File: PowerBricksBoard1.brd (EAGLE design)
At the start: 75.6 x 50.8 mm, 16 parts

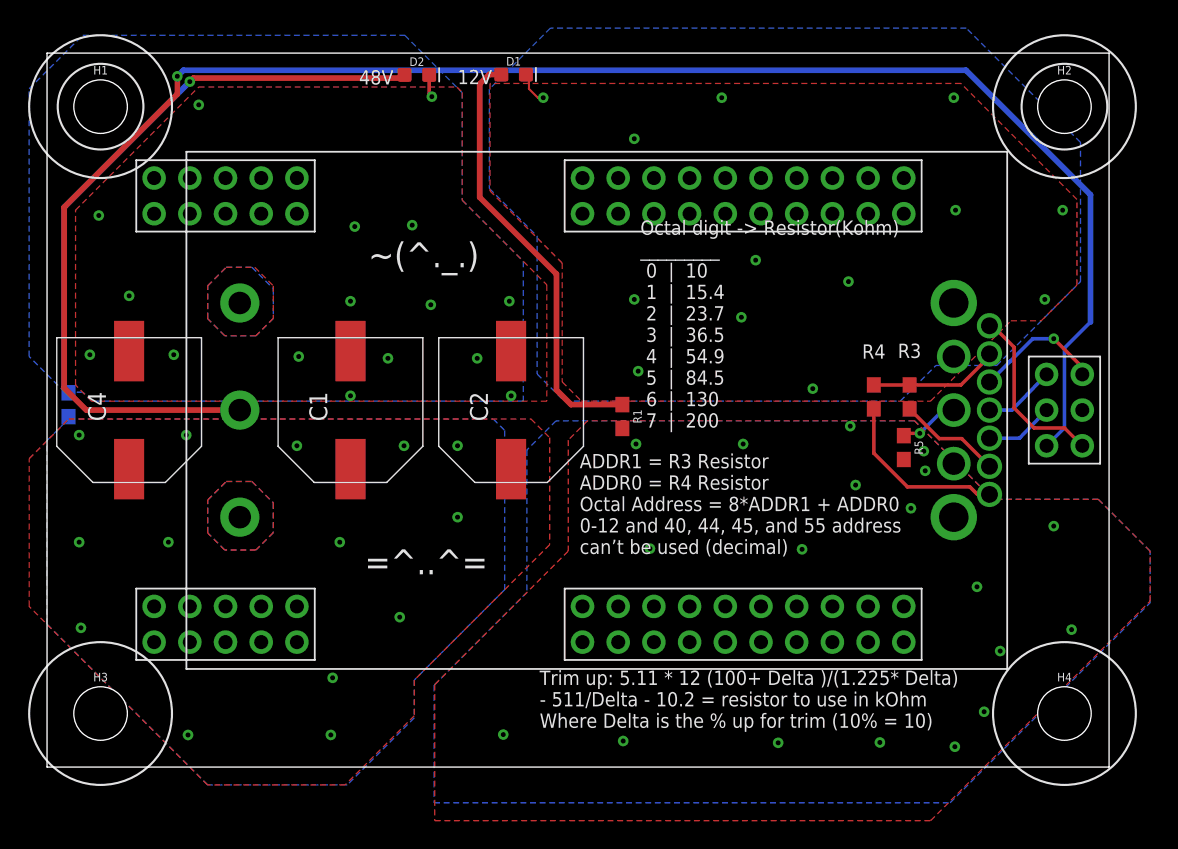
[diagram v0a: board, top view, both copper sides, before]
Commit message: 50mil smol
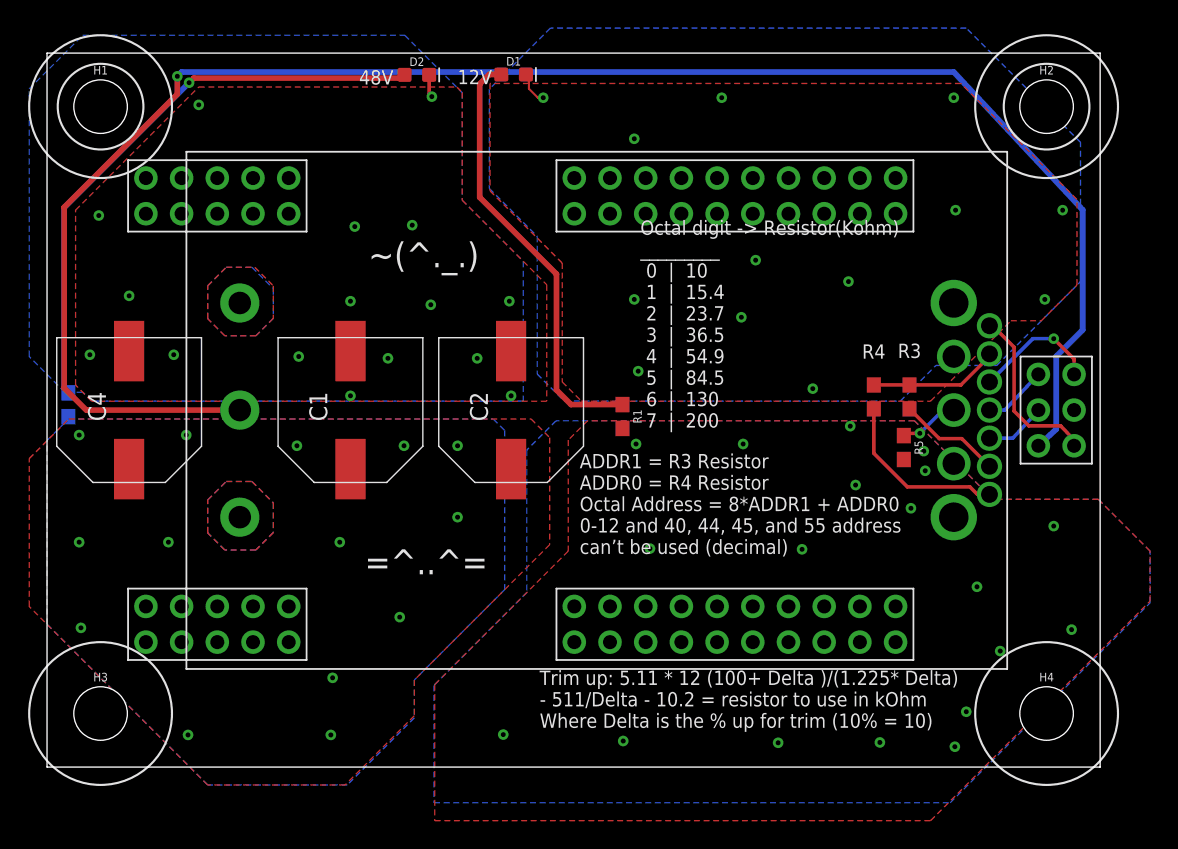
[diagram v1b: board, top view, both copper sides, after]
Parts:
- moved H2 1.27 mm to (71.1, 47.0)
- moved H4 1.27 mm to (71.1, 3.81)
- moved U$1 0.58 mm to (37.5, 25.4)
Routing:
- net ON/OFF: track 126.6 -> 125.6 mm
- net ALERT: track 5.14 -> 4.58 mm
- net CLK: track 4.92 -> 4.37 mm
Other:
- board size 75.6 x 50.8 mm -> 74.9 x 50.8 mm

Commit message: Revert "trim"
This reverts commit 0055e3f947d82e2e184832a38c8fbe8e78d74489.
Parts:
- R5: value 510k -> 475k
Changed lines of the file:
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@@
 <attribute name="VALUE" x="58.0644" y="26.3398" size="0.6096" layer="27" font="vector" ratio="20" rot="R270" align="top-center"/>
 </element>
-<element name="R5" library="SparkFun-Resistors" library_urn="urn:adsk.eagle:library:532" package="0603" package3d_urn="urn:adsk.eagle:package:39650/1" value="510k" x="60.96" y="22.733" smashed="yes" rot="R270">
+<element name="R5" library="SparkFun-Resistors" library_urn="urn:adsk.eagle:library:532" package="0603" package3d_urn="urn:adsk.eagle:package:39650/1" value="475k" x="60.96" y="22.733" smashed="yes" rot="R270">
 <attribute name="NAME" x="61.721996875" y="22.733003125" size="0.6096" layer="25" font="vector" ratio="20" rot="R270" align="bottom-center"/>
 <attribute name="PROD_ID" value=" " x="-30.479996875" y="-64.896996875" size="1.778" layer="27" rot="R270" display="off"/>

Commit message: Revert "Revert "trim""
This reverts commit 46b5d4a1c2a012013371b894087438f3b54206c6.
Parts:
- R5: value 475k -> 510k
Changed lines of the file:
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@@
 <attribute name="VALUE" x="58.0644" y="26.3398" size="0.6096" layer="27" font="vector" ratio="20" rot="R270" align="top-center"/>
 </element>
-<element name="R5" library="SparkFun-Resistors" library_urn="urn:adsk.eagle:library:532" package="0603" package3d_urn="urn:adsk.eagle:package:39650/1" value="475k" x="60.96" y="22.733" smashed="yes" rot="R270">
+<element name="R5" library="SparkFun-Resistors" library_urn="urn:adsk.eagle:library:532" package="0603" package3d_urn="urn:adsk.eagle:package:39650/1" value="510k" x="60.96" y="22.733" smashed="yes" rot="R270">
 <attribute name="NAME" x="61.721996875" y="22.733003125" size="0.6096" layer="25" font="vector" ratio="20" rot="R270" align="bottom-center"/>
 <attribute name="PROD_ID" value=" " x="-30.479996875" y="-64.896996875" size="1.778" layer="27" rot="R270" display="off"/>

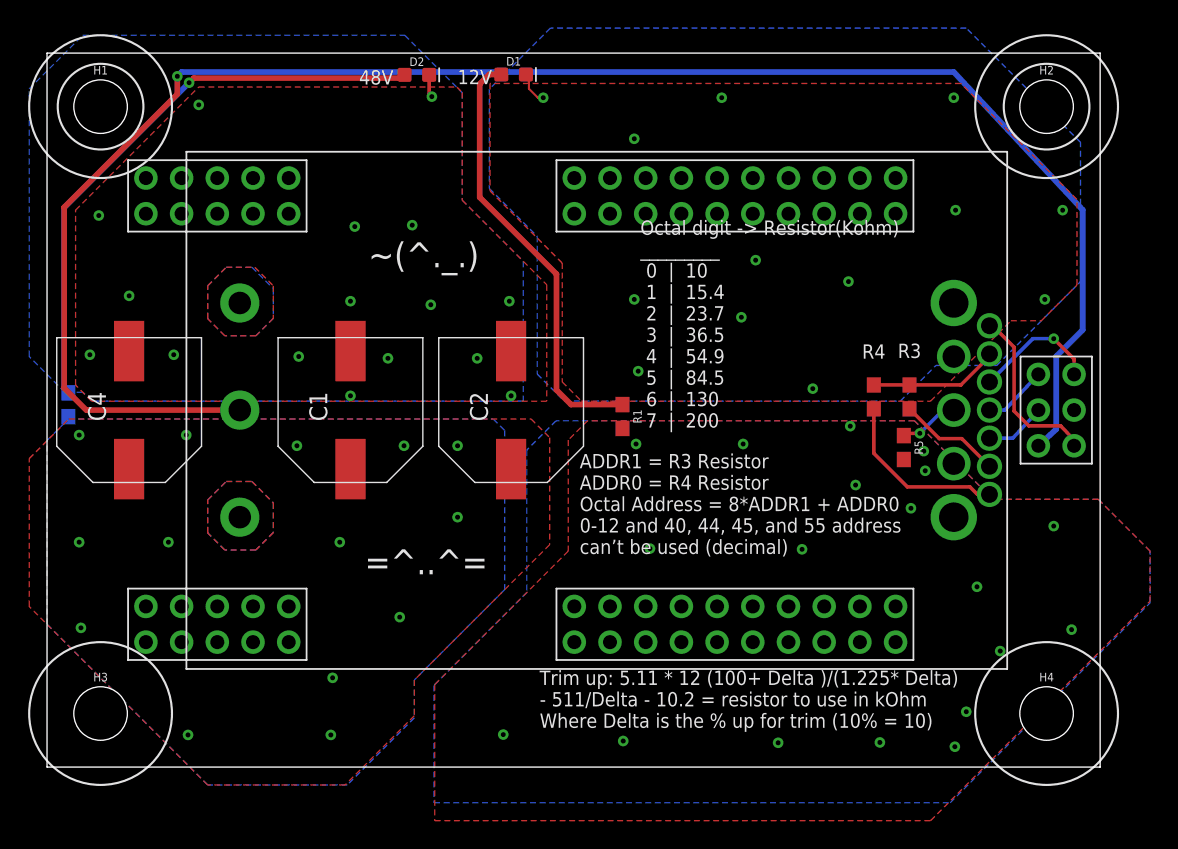
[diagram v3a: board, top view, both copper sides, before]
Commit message: euhreiuhthjtrgrefwefrgyjgr
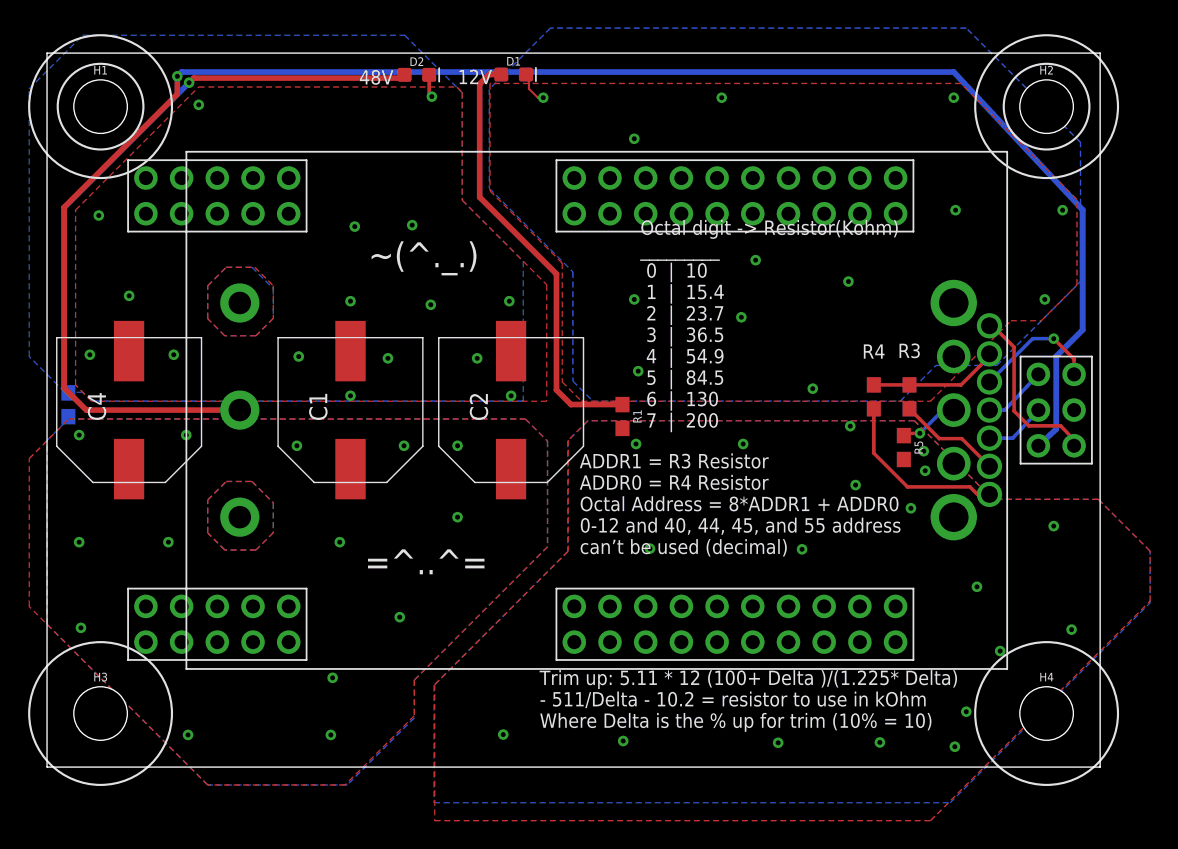
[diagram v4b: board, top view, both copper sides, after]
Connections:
- net 48V_GND renamed 48V
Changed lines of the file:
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@@
 </elements>
 <signals>
-<signal name="48V_GND">
-<contactref element="C1" pad="+"/>
-<contactref element="C2" pad="+"/>
-<contactref element="C4" pad="+"/>
-<contactref element="R2" pad="2"/>
-<contactref element="U$2" pad="1"/>
-<polygon width="0.9144" layer="1" isolate="0.508" rank="2">
-<vertex x="1.5494" y="24.765"/>
-<vertex x="34.4424" y="24.765"/>
-<vertex x="35.7632" y="23.4442"/>
-<vertex x="35.7632" y="15.8242"/>
-<vertex x="26.1366" y="6.1976"/>
-<vertex x="26.1366" y="3.6576"/>
-<vertex x="21.209" y="-1.27"/>
-<vertex x="11.43" y="-1.27"/>
-<vertex x="-1.27" y="11.43"/>
-<vertex x="-1.27" y="21.9456"/>
-</polygon>
-<polygon width="0.9144" layer="16" isolate="0.508" rank="2">
-<vertex x="1.524" y="24.765"/>
-<vertex x="31.75" y="24.765"/>
-<vertex x="32.5628" y="23.9522"/>
-<vertex x="32.5628" y="12.6238"/>
-<vertex x="26.1366" y="6.1976"/>
-<vertex x="26.1366" y="3.5052"/>
-<vertex x="21.3614" y="-1.27"/>
-<vertex x="11.43" y="-1.27"/>
-<vertex x="0" y="10.16"/>
-<vertex x="0" y="23.241"/>
-</polygon>
-<via x="17.78" y="22.86" extent="1-16" drill="0.35"/>
-<via x="25.4" y="22.86" extent="1-16" drill="0.35"/>
-<via x="29.21" y="22.86" extent="1-16" drill="0.35"/>
-<via x="25.0952" y="10.668" extent="1-16" drill="0.35"/>
-<via x="20.32" y="6.35" extent="1-16" drill="0.35"/>
-<via x="29.21" y="17.78" extent="1-16" drill="0.35"/>
-<via x="20.828" y="16.002" extent="1-16" drill="0.35"/>
-<via x="20.193" y="2.286" extent="1-16" drill="0.35"/>
-<via x="10.033" y="2.286" extent="1-16" drill="0.35"/>
-<via x="2.413" y="9.906" extent="1-16" drill="0.35"/>
-<via x="2.286" y="23.622" extent="1-16" drill="0.35"/>
-<via x="9.906" y="23.622" extent="1-16" drill="0.35"/>
-<via x="2.286" y="16.002" extent="1-16" drill="0.35"/>
-<via x="8.636" y="16.002" extent="1-16" drill="0.35"/>
-<contactref element="U$1" pad="1@1"/>
-<contactref element="U$1" pad="1@5"/>
-<contactref element="U$1" pad="1@6"/>
-<contactref element="U$1" pad="1@9"/>
-<contactref element="U$1" pad="1@10"/>
-<contactref element="U$1" pad="1@4"/>
-<contactref element="U$1" pad="1@3"/>
-<contactref element="U$1" pad="1@2"/>
-<contactref element="U$1" pad="1@8"/>
-<contactref element="U$1" pad="1@7"/>
-<polygon width="0.1524" layer="1" thermals="no">
-<vertex x="12.7508" y="20.32"/>
-<vertex x="14.5796" y="20.32"/>
-<vertex x="16.1036" y="18.796"/>
-<vertex x="16.1036" y="16.6878"/>
-<vertex x="14.859" y="15.4432"/>
-<vertex x="12.6492" y="15.4432"/>
-<vertex x="11.43" y="16.6624"/>
-<vertex x="11.43" y="18.9992"/>
-</polygon>
-<polygon width="0.1524" layer="16" thermals="no">
-<vertex x="12.7508" y="20.32"/>
-<vertex x="14.5796" y="20.32"/>
-<vertex x="16.1036" y="18.796"/>
-<vertex x="16.1036" y="16.6878"/>
-<vertex x="14.859" y="15.4432"/>
-<vertex x="12.6492" y="15.4432"/>
-<vertex x="11.43" y="16.6624"/>
-<vertex x="11.43" y="18.9992"/>
-</polygon>
-</signal>
 <signal name="48_GND">
 <contactref element="C1" pad="-"/>
@@
 <contactref element="U$2" pad="9"/>
 <polygon width="0.9144" layer="16" isolate="0.508">
-<vertex x="34.1376" y="12.4206"/>
+<vertex x="37.0586" y="15.3416"/>
 <vertex x="27.5336" y="5.8166"/>
 <vertex x="27.5336" y="-2.54"/>
@@
 <vertex x="67.31" y="19.05"/>
 <vertex x="61.722" y="24.638"/>
-<vertex x="36.2204" y="24.638"/>
-<vertex x="34.1376" y="22.5552"/>
+<vertex x="38.5064" y="24.638"/>
+<vertex x="37.0586" y="23.1902"/>
 </polygon>
 <polygon width="0.9144" layer="1" isolate="0.508">
@@
 <vertex x="31.4706" y="48.2346"/>
 <vertex x="31.4706" y="41.1734"/>
-<vertex x="34.8742" y="37.7698"/>
-<vertex x="34.8742" y="27.9654"/>
-<vertex x="36.8046" y="26.035"/>
+<vertex x="37.4142" y="35.2298"/>
+<vertex x="37.4142" y="27.4574"/>
+<vertex x="38.8366" y="26.035"/>
 <vertex x="60.706" y="26.035"/>
 <vertex x="63.246" y="28.575"/>
@@
 <wire x1="71.8058" y1="24.037071875" x2="71.8058" y2="29.22189375" width="0.4064" layer="16"/>
 </signal>
+<signal name="48V">
+<contactref element="U$2" pad="1"/>
+<contactref element="U$1" pad="1@1"/>
+<contactref element="U$1" pad="1@5"/>
+<contactref element="U$1" pad="1@6"/>
+<contactref element="U$1" pad="1@9"/>
+<contactref element="U$1" pad="1@10"/>
+<contactref element="U$1" pad="1@4"/>
+<contactref element="U$1" pad="1@3"/>
+<contactref element="U$1" pad="1@2"/>
+<contactref element="U$1" pad="1@8"/>
+<contactref element="U$1" pad="1@7"/>
+<contactref element="C1" pad="+"/>
+<contactref element="C2" pad="+"/>
+<contactref element="C4" pad="+"/>
+<contactref element="R2" pad="2"/>
+<polygon width="0.9144" layer="1" isolate="0.508" rank="2">
+<vertex x="1.5494" y="24.765"/>
+<vertex x="34.036" y="24.765"/>
+<vertex x="35.6108" y="23.1902"/>
+<vertex x="35.6108" y="15.6718"/>
+<vertex x="26.1366" y="6.1976"/>
+<vertex x="26.1366" y="3.6576"/>
+<vertex x="21.209" y="-1.27"/>
+<vertex x="11.43" y="-1.27"/>
+<vertex x="-1.27" y="11.43"/>
+<vertex x="-1.27" y="21.9456"/>
+</polygon>
+<polygon width="0.9144" layer="16" isolate="0.508" rank="2">
+<vertex x="1.524" y="24.765"/>
+<vertex x="34.036" y="24.765"/>
+<vertex x="35.6108" y="23.1902"/>
+<vertex x="35.6108" y="15.6718"/>
+<vertex x="26.1366" y="6.1976"/>
+<vertex x="26.1366" y="3.5052"/>
+<vertex x="21.3614" y="-1.27"/>
+<vertex x="11.43" y="-1.27"/>
+<vertex x="0" y="10.16"/>
+<vertex x="0" y="23.241"/>
+</polygon>
+<via x="17.78" y="22.86" extent="1-16" drill="0.35"/>
+<via x="25.4" y="22.86" extent="1-16" drill="0.35"/>
+<via x="29.21" y="22.86" extent="1-16" drill="0.35"/>
+<via x="25.0952" y="10.668" extent="1-16" drill="0.35"/>
+<via x="20.32" y="6.35" extent="1-16" drill="0.35"/>
+<via x="29.21" y="17.78" extent="1-16" drill="0.35"/>
+<via x="20.828" y="16.002" extent="1-16" drill="0.35"/>
+<via x="20.193" y="2.286" extent="1-16" drill="0.35"/>
+<via x="10.033" y="2.286" extent="1-16" drill="0.35"/>
+<via x="2.413" y="9.906" extent="1-16" drill="0.35"/>
+<via x="2.286" y="23.622" extent="1-16" drill="0.35"/>
+<via x="9.906" y="23.622" extent="1-16" drill="0.35"/>
+<via x="2.286" y="16.002" extent="1-16" drill="0.35"/>
+<via x="8.636" y="16.002" extent="1-16" drill="0.35"/>
+<polygon width="0.1524" layer="1" thermals="no">
+<vertex x="12.7508" y="20.32"/>
+<vertex x="14.5796" y="20.32"/>
+<vertex x="16.1036" y="18.796"/>
+<vertex x="16.1036" y="16.6878"/>
+<vertex x="14.859" y="15.4432"/>
+<vertex x="12.6492" y="15.4432"/>
+<vertex x="11.43" y="16.6624"/>
+<vertex x="11.43" y="18.9992"/>
+</polygon>
+<polygon width="0.1524" layer="16" thermals="no">
+<vertex x="12.7508" y="20.32"/>
+<vertex x="14.5796" y="20.32"/>
+<vertex x="16.1036" y="18.796"/>
+<vertex x="16.1036" y="16.6878"/>
+<vertex x="14.859" y="15.4432"/>
+<vertex x="12.6492" y="15.4432"/>
+<vertex x="11.43" y="16.6624"/>
+<vertex x="11.43" y="18.9992"/>
+</polygon>
+</signal>
 </signals>
